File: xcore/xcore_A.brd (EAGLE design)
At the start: 80 x 80 mm, 37 parts, among them U1 NC7WZ07, X1 XEF216-512-TQ128

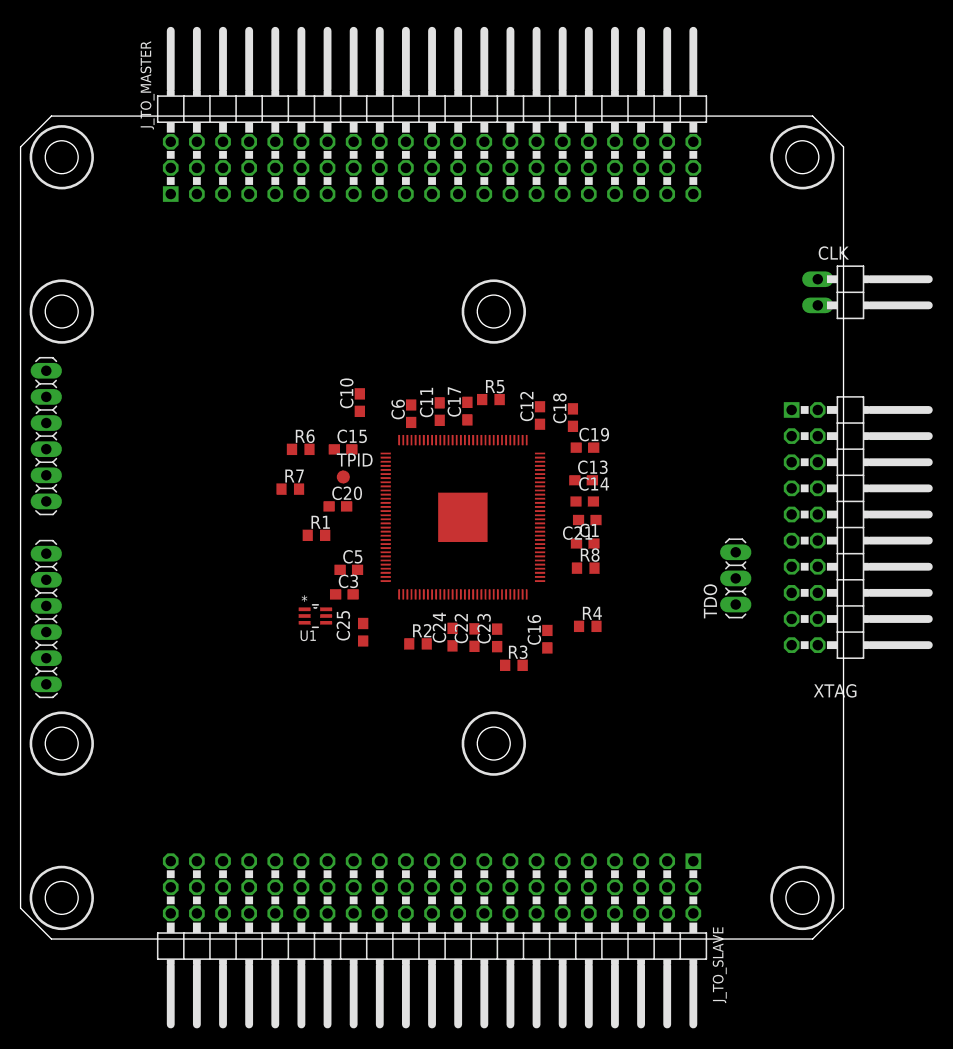
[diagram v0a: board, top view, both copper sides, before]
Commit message: xcore: WIP PCB
Signed-off-by: malo <pavol.malosek@gmail.com>
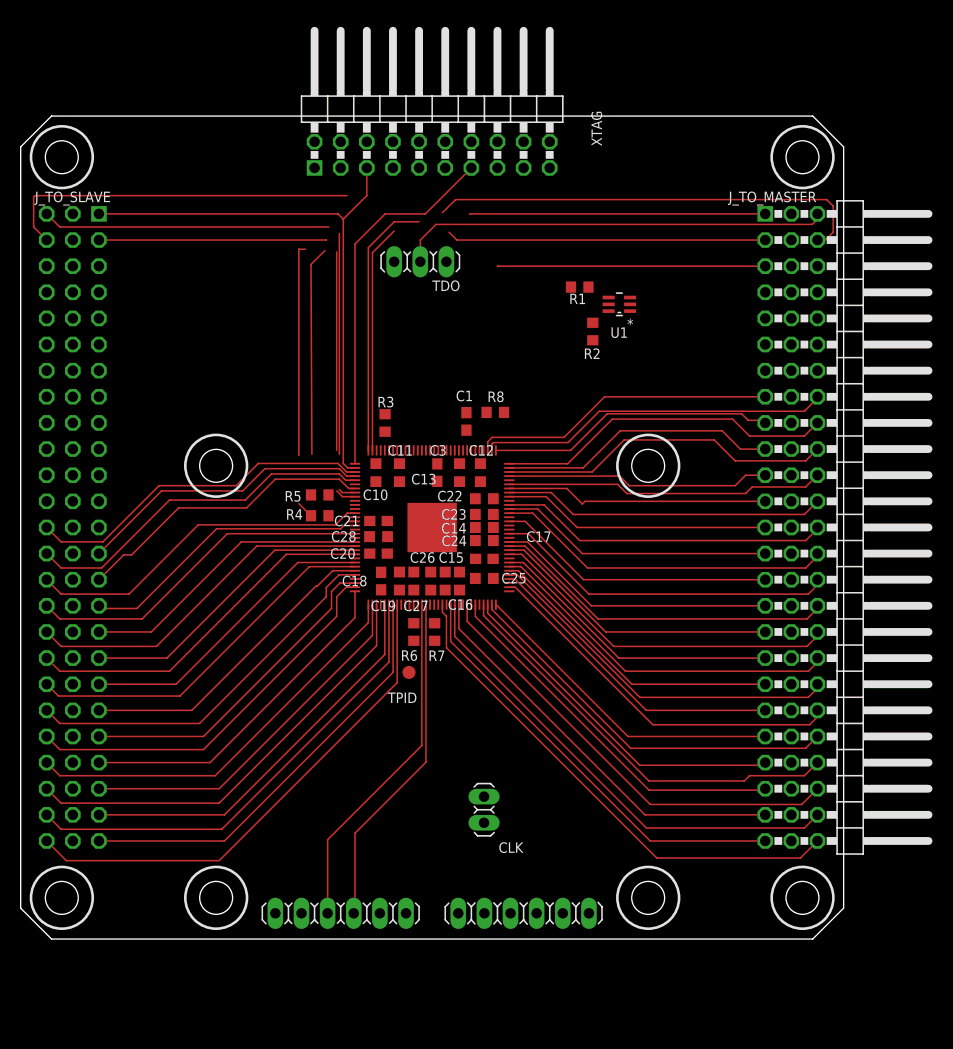
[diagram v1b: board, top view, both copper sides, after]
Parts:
- removed C5, C6: 100n, 0603, rcl:C0603
- added C26, C27, C28: 100n, 0603, rcl:C0603K
- C10, C11, C12, C13, C14, C16, C17, C18, C22, C23, C24, C25: device rcl:C0603 -> rcl:C0603K
- CLK: device 25pinhead:1X02/90 -> 25pinhead:1X02
- J_TO_MASTER, J_TO_SLAVE: value TSW-121-08-G-T-RA -> TSW-125-08-G-T-RA; device 25pinhead:3X21/90 -> 25pinhead:3X25/90
- moved PWR 80.0 mm to (0.01, 80.0), turned to 270 degrees
- moved CLK 62.0 mm to (45.1, 12.6), turned to 90 degrees
- moved XTAG 58.4 mm to (40.0, 81.3), turned to 0 degrees
- moved J_TO_SLAVE 55.8 mm to (2.54, 40.0), flipped to the bottom, turned to 270 degrees
- moved J_TO_MASTER 55.8 mm to (77.5, 40.0), turned to 270 degrees
- moved TDO 43.5 mm to (38.9, 65.8), turned to 180 degrees
- moved U1 42.3 mm to (58.2, 61.7), turned to 180 degrees
- moved R1 35.2 mm to (54.4, 63.4), turned to 180 degrees
- moved R2 34.8 mm to (55.6, 59.1), turned to 270 degrees
- moved R4 28.2 mm to (29.1, 41.1)
- moved R3 26.7 mm to (35.4, 50.2), turned to 270 degrees
- moved C19 23.7 mm to (35.1, 34.8), turned to 270 degrees
- moved C18 23.2 mm to (36.8, 34.8), turned to 270 degrees
- moved R6 20.9 mm to (38.2, 29.8), turned to 90 degrees
- moved C21 20.3 mm to (34.8, 40.6)
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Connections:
- net N$1 renamed X0D43
- net N$11 renamed PLL_AVDD
- net N$2 renamed IO1
- net N$3 renamed X0D42
- net N$7 renamed USB_RTUNE
- new net X0D02: J_TO_SLAVE.70, X1.37
- new net X0D03: J_TO_SLAVE.72, X1.38
- new net X0D08: J_TO_SLAVE.73, X1.39
- new net X0D09: J_TO_SLAVE.75, X1.40
- new net X0D14: J_TO_MASTER.69, X1.57
- new net X0D15: X1.58
- new net X0D16: J_TO_MASTER.58, X1.68
- new net X0D17: J_TO_MASTER.57, X1.69
- new net X0D18: J_TO_MASTER.55, X1.70
- new net X0D19: J_TO_MASTER.54, X1.71
- new net X0D20: J_TO_MASTER.67, X1.59
- new net X0D21: J_TO_MASTER.66, X1.61
- new net X0D26: J_TO_MASTER.31, X1.93
- new net X0D27: J_TO_MASTER.30, X1.94
- new net X0D28: J_TO_MASTER.27, X1.96
- new net X0D29: J_TO_MASTER.24, X1.98
- new net X0D30: J_TO_MASTER.22, X1.99
- new net X0D31: J_TO_MASTER.21, X1.100
- new net X0D32: J_TO_MASTER.28, X1.95
- new net X0D33: J_TO_MASTER.25, X1.97
- new net X1D02: J_TO_MASTER.52, X1.72
- new net X1D03: J_TO_MASTER.51, X1.74
- new net X1D04: J_TO_MASTER.49, X1.75
- new net X1D05: J_TO_MASTER.48, X1.76
- new net X1D06: J_TO_MASTER.46, X1.77
- new net X1D07: J_TO_MASTER.45, X1.79
- new net X1D08: J_TO_MASTER.43, X1.82
- new net X1D09: J_TO_MASTER.42, X1.84
- new net X1D14: J_TO_MASTER.75, X1.51
- new net X1D15: J_TO_MASTER.73, X1.53
- new net X1D16: J_TO_SLAVE.52, X1.22
- new net X1D17: J_TO_SLAVE.54, X1.23
- new net X1D18: J_TO_SLAVE.55, X1.25
- new net X1D19: J_TO_SLAVE.57, X1.26
- new net X1D20: J_TO_MASTER.72, X1.54
- new net X1D21: J_TO_MASTER.70, X1.55
- new net X1D26: J_TO_MASTER.13, X1.112
- new net X1D27: J_TO_MASTER.12, X1.113
- new net X1D28: J_TO_MASTER.10, X1.114
- new net X1D29: J_TO_MASTER.9, X1.115
- new net X1D30: J_TO_SLAVE.30, X1.116
- new net X1D31: J_TO_SLAVE.31, X1.117
- new net X1D32: J_TO_SLAVE.33, X1.118
- new net X1D33: J_TO_SLAVE.34, X1.119
- new net X1D40: J_TO_MASTER.19, X1.106
- new net X1D41: J_TO_MASTER.18, X1.107
- new net X1D42: J_TO_MASTER.16, X1.108
- new net X1D43: J_TO_MASTER.15, X1.109
- net +3V3: now also C26.2, C27.2, C28.2; no longer C5.2, C6.2
- net GND: now also C26.1, C27.1, C28.1, J_TO_MASTER.65, J_TO_MASTER.68, J_TO_MASTER.71, J_TO_MASTER.74, J_TO_SLAVE.65, J_TO_SLAVE.68, J_TO_SLAVE.71, J_TO_SLAVE.74; no longer C5.1, C6.1
- net TCK: now also J_TO_MASTER.6, J_TO_SLAVE.6; no longer J_TO_MASTER.60, J_TO_SLAVE.60
- net TDI: now also J_TO_MASTER.1, J_TO_SLAVE.1; no longer J_TO_MASTER.51, J_TO_SLAVE.51
- net TDO_IN: now also J_TO_SLAVE.3; no longer J_TO_SLAVE.54
- net TDO_OUT: now also J_TO_MASTER.3; no longer J_TO_MASTER.54
- net TMS: now also J_TO_MASTER.4, J_TO_SLAVE.4; no longer J_TO_MASTER.57, J_TO_SLAVE.57
- net X0D00: now also J_TO_SLAVE.61; no longer J_TO_MASTER.1
- net X0D01: now also J_TO_SLAVE.58; no longer J_TO_MASTER.4
- net X0D04: now also J_TO_SLAVE.63; no longer J_TO_MASTER.12
- net X0D05: now also J_TO_SLAVE.66; no longer J_TO_MASTER.15
- net X0D06: now also J_TO_SLAVE.67; no longer J_TO_MASTER.18
- net X0D07: now also J_TO_SLAVE.69; no longer J_TO_MASTER.21
- net X0D10: now also J_TO_SLAVE.60; no longer J_TO_MASTER.7
- net X0D11: now also J_TO_SLAVE.64; no longer J_TO_MASTER.10
- net X0D12: now also J_TO_MASTER.64; no longer J_TO_MASTER.13
- net X0D13: now also J_TO_MASTER.63; no longer J_TO_MASTER.16
- net X0D22: now also J_TO_MASTER.61; no longer J_TO_MASTER.19
- net X0D23: now also J_TO_MASTER.60; no longer J_TO_MASTER.22
- net X0D24: now also J_TO_MASTER.37; no longer J_TO_MASTER.25
- net X0D25: now also J_TO_MASTER.36; no longer J_TO_MASTER.28
- net X0D34: now also J_TO_MASTER.34; no longer J_TO_MASTER.31
- net X0D35: now also J_TO_MASTER.33; no longer J_TO_MASTER.34
- net X0D36: now also J_TO_SLAVE.39; no longer J_TO_MASTER.37
- net X0D37: now also J_TO_SLAVE.40; no longer J_TO_MASTER.3
- net X0D38: now also J_TO_SLAVE.42; no longer J_TO_MASTER.6
- net X0D39: now also J_TO_SLAVE.43; no longer J_TO_MASTER.9
- net X1D00: now also J_TO_MASTER.40; no longer J_TO_SLAVE.1
- net X1D01: now also J_TO_MASTER.39; no longer J_TO_SLAVE.4
- net X1D10: now also J_TO_SLAVE.36; no longer J_TO_SLAVE.7
- net X1D11: now also J_TO_SLAVE.37; no longer J_TO_SLAVE.10
- net X1D35: now also J_TO_SLAVE.45; no longer J_TO_SLAVE.13
- net X1D36: now also J_TO_SLAVE.46; no longer J_TO_SLAVE.16
- net X1D37: now also J_TO_SLAVE.48; no longer J_TO_SLAVE.19
- net X1D38: now also J_TO_SLAVE.49; no longer J_TO_SLAVE.22, J_TO_SLAVE.25
- net X1D39: now also J_TO_SLAVE.51
- net XSYS_RST_N: now also J_TO_MASTER.7, J_TO_SLAVE.7; no longer J_TO_MASTER.63, J_TO_SLAVE.63
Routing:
- net TCK: track 0.00 -> 104.1 mm
- net TDI: track 0.00 -> 83.7 mm
- net TMS: track 0.00 -> 75.4 mm
- net X0D09: track 0.00 -> 49.6 mm
- net X1D14: track 0.00 -> 49.6 mm
- net X1D20: track 0.00 -> 46.6 mm
- net X0D03: track 0.00 -> 46.2 mm
- net X0D14: track 0.00 -> 43.7 mm
- net X0D07: track 0.00 -> 43.0 mm
- net X1D15: track 0.00 -> 42.2 mm
- net TDO_OUT: track 0.00 -> 42.1 mm
- net X0D08: track 0.00 -> 42.0 mm
- net X0D21: track 0.00 -> 40.9 mm
- net X0D05: track 0.00 -> 39.7 mm
- net X1D21: track 0.00 -> 39.6 mm
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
